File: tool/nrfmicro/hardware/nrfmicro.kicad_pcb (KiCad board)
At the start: 2 copper layers, 17.2 x 33.3 mm, 25 parts, among them J1 USB-C Conn, J2 SWD, J3 Ex_Bat, J4 Ex_USB, J5 , J6 , Q1 AO3407, Q2 AO3407, U1 E73-2G4M08S1C, U2 XC6220B331MR-G, U3 TP4054, U4 ProMicro, X1 32.768kHz

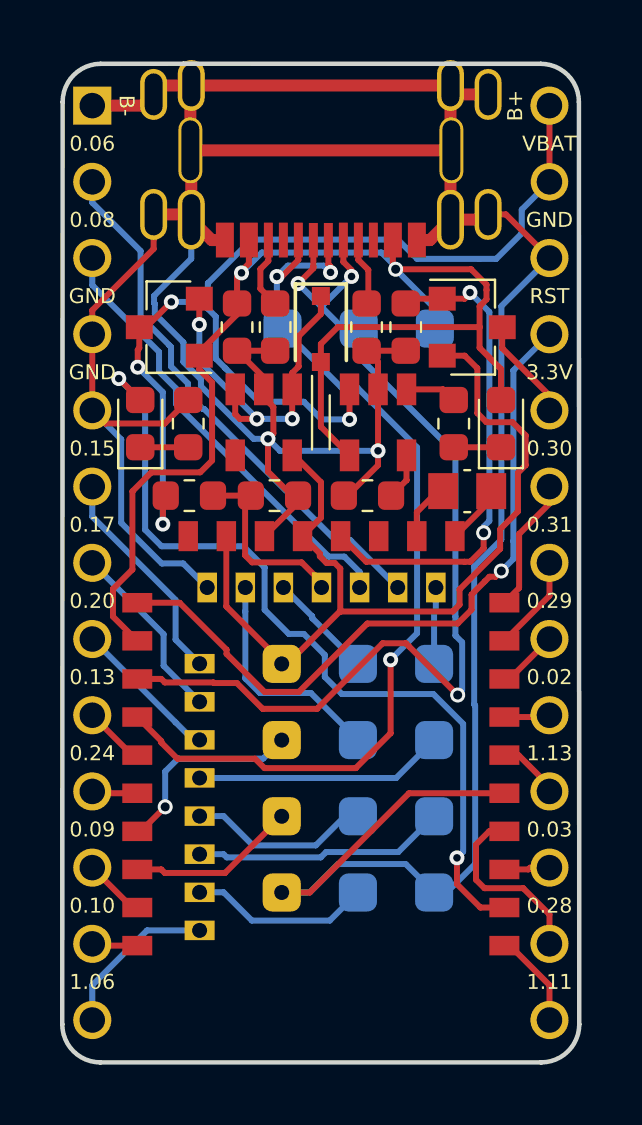
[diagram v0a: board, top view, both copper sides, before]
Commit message: update 13:33 24/01/2021
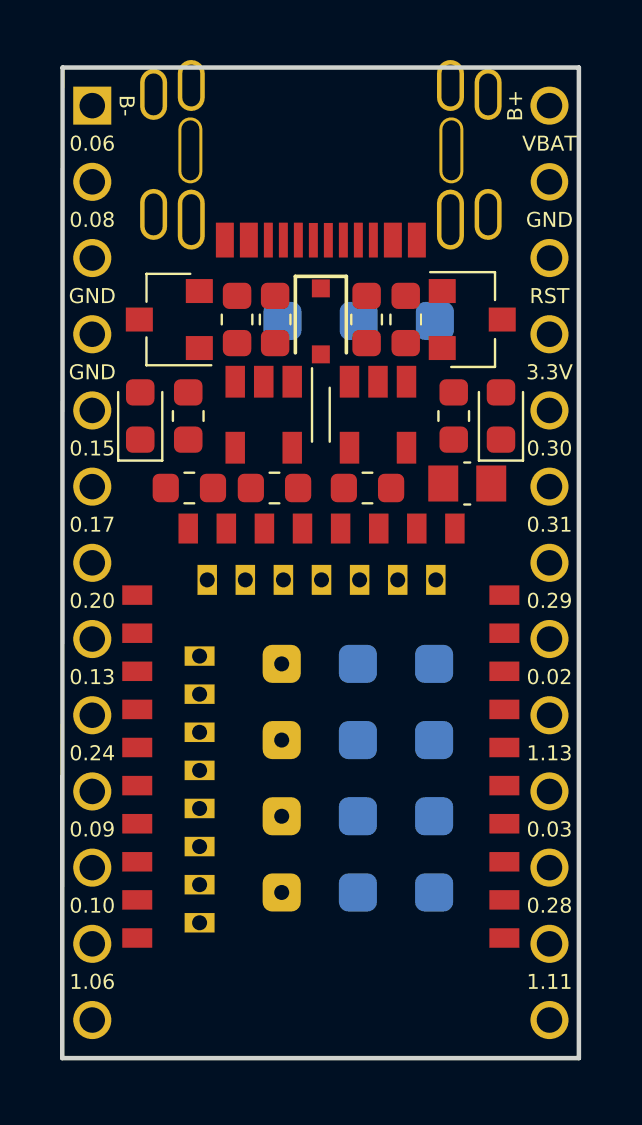
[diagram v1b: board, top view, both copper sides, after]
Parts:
- moved X1 0.25 mm to (32.6, 32.6)
- moved D2 0.25 mm to (21.7, 30.3)
- moved D3 0.25 mm to (33.7, 30.3)
- moved R1 0.25 mm to (24.9, 27.1)
- moved R2 0.25 mm to (26.2, 27.1)
- moved R3 0.25 mm to (29.2, 27.1)
- moved R4 0.25 mm to (23.3, 30.3)
- moved R8 0.25 mm to (32.1, 30.3)
- moved R9 0.25 mm to (30.6, 27.1)
- moved D1 0.25 mm to (27.7, 27.2)
- moved J4 0.25 mm to (27.7, 27.2)
- moved Q1 0.25 mm to (22.7, 27.1)
- moved Q2 0.25 mm to (32.8, 27.1)
- moved R5 0.25 mm to (29.3, 32.7)
- moved R6 0.25 mm to (23.3, 32.7)
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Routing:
- net GND: track 128.7 -> 0.00 mm, vias 2 -> 0
- net VBUS: track 43.3 -> 0.00 mm, vias 2 -> 0
- net VBAT: track 35.8 -> 0.00 mm, vias 4 -> 0
- net DATA-: track 33.5 -> 0.00 mm, vias 3 -> 0
- net DATA+: track 32.2 -> 0.00 mm, vias 3 -> 0
- net nRF_VDD: track 29.6 -> 0.00 mm
- net BLUE_LED: track 28.3 -> 0.00 mm, vias 2 -> 0
- net RESET: track 24.0 -> 0.00 mm, vias 1 -> 0
- net /P0.06: track 18.1 -> 0.00 mm
- net POWER_PIN: track 16.5 -> 0.00 mm, vias 2 -> 0
- net /P0.08: track 15.0 -> 0.00 mm
- net Net-(D1-Pad1): track 12.1 -> 0.00 mm, vias 3 -> 0
- net /P1.02: track 8.43 -> 0.00 mm
- net /P0.22: track 8.34 -> 0.00 mm
- net /P0.07: track 7.64 -> 0.00 mm
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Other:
- board size 17.2 x 33.3 mm -> 17.2 x 33 mm

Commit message: update 17:18 28/01/2021
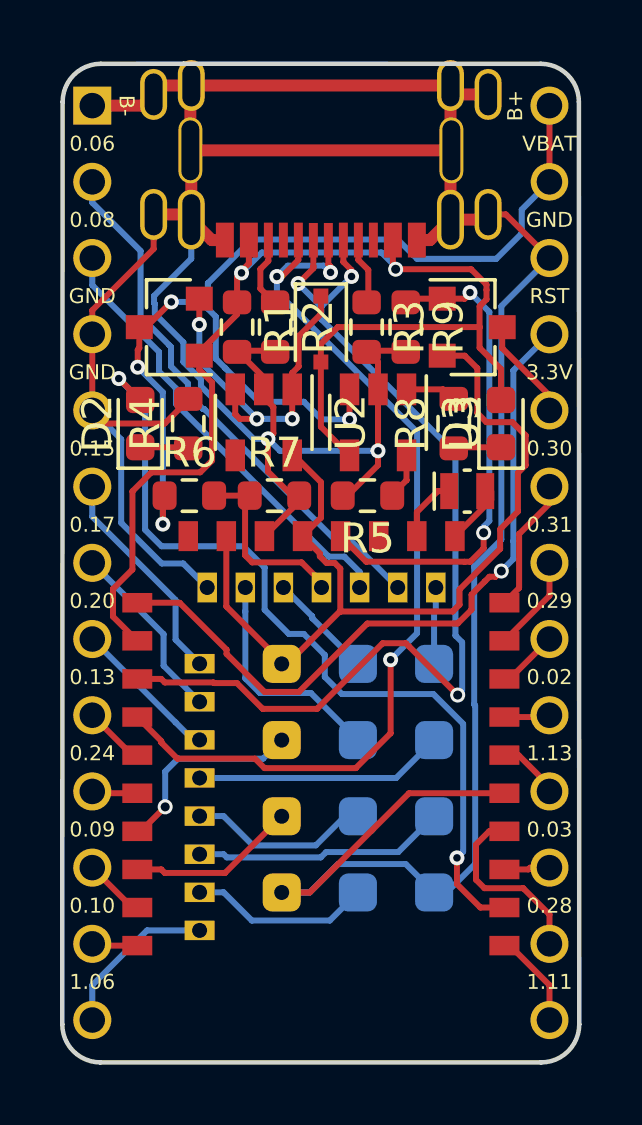
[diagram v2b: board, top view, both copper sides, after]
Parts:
- removed J4: Ex_USB, nrfmicro:connector_usb
- moved X1 0.25 mm to (32.6, 32.9)
- moved D2 0.25 mm to (21.7, 30.6)
- moved D3 0.25 mm to (33.7, 30.6)
- moved R1 0.25 mm to (24.9, 27.4)
- moved R2 0.25 mm to (26.2, 27.4)
- moved R3 0.25 mm to (29.2, 27.4)
- moved R4 0.25 mm to (23.3, 30.6)
- moved R8 0.25 mm to (32.1, 30.6)
- moved R9 0.25 mm to (30.6, 27.4)
- moved D1 0.25 mm to (27.7, 27.4)
- moved Q1 0.25 mm to (22.7, 27.4)
- moved Q2 0.25 mm to (32.8, 27.4)
- moved R5 0.25 mm to (29.3, 33.0)
- moved R6 0.25 mm to (23.3, 33.0)
- moved R7 0.25 mm to (26.2, 33.0)
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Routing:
- net GND: track 0.00 -> 128.7 mm, vias 0 -> 2
- net VBUS: track 0.00 -> 40.8 mm, vias 0 -> 2
- net VBAT: track 0.00 -> 35.8 mm, vias 0 -> 4
- net DATA-: track 0.00 -> 33.2 mm, vias 0 -> 3
- net DATA+: track 0.00 -> 31.9 mm, vias 0 -> 3
- net nRF_VDD: track 0.00 -> 29.6 mm
- net BLUE_LED: track 0.00 -> 28.3 mm, vias 0 -> 2
- net RESET: track 0.00 -> 24.0 mm, vias 0 -> 1
- net /P0.06: track 0.00 -> 18.1 mm
- net POWER_PIN: track 0.00 -> 16.5 mm, vias 0 -> 2
- net /P0.08: track 0.00 -> 15.0 mm
- net Net-(D1-Pad1): track 0.00 -> 12.1 mm, vias 0 -> 3
- net /P1.02: track 0.00 -> 8.43 mm
- net /P0.22: track 0.00 -> 8.34 mm
- net /P0.07: track 0.00 -> 7.64 mm
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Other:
- board size 17.2 x 33 mm -> 17.2 x 33.3 mm
